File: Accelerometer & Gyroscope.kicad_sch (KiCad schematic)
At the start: 5 parts, among them U9 LSM6DS3

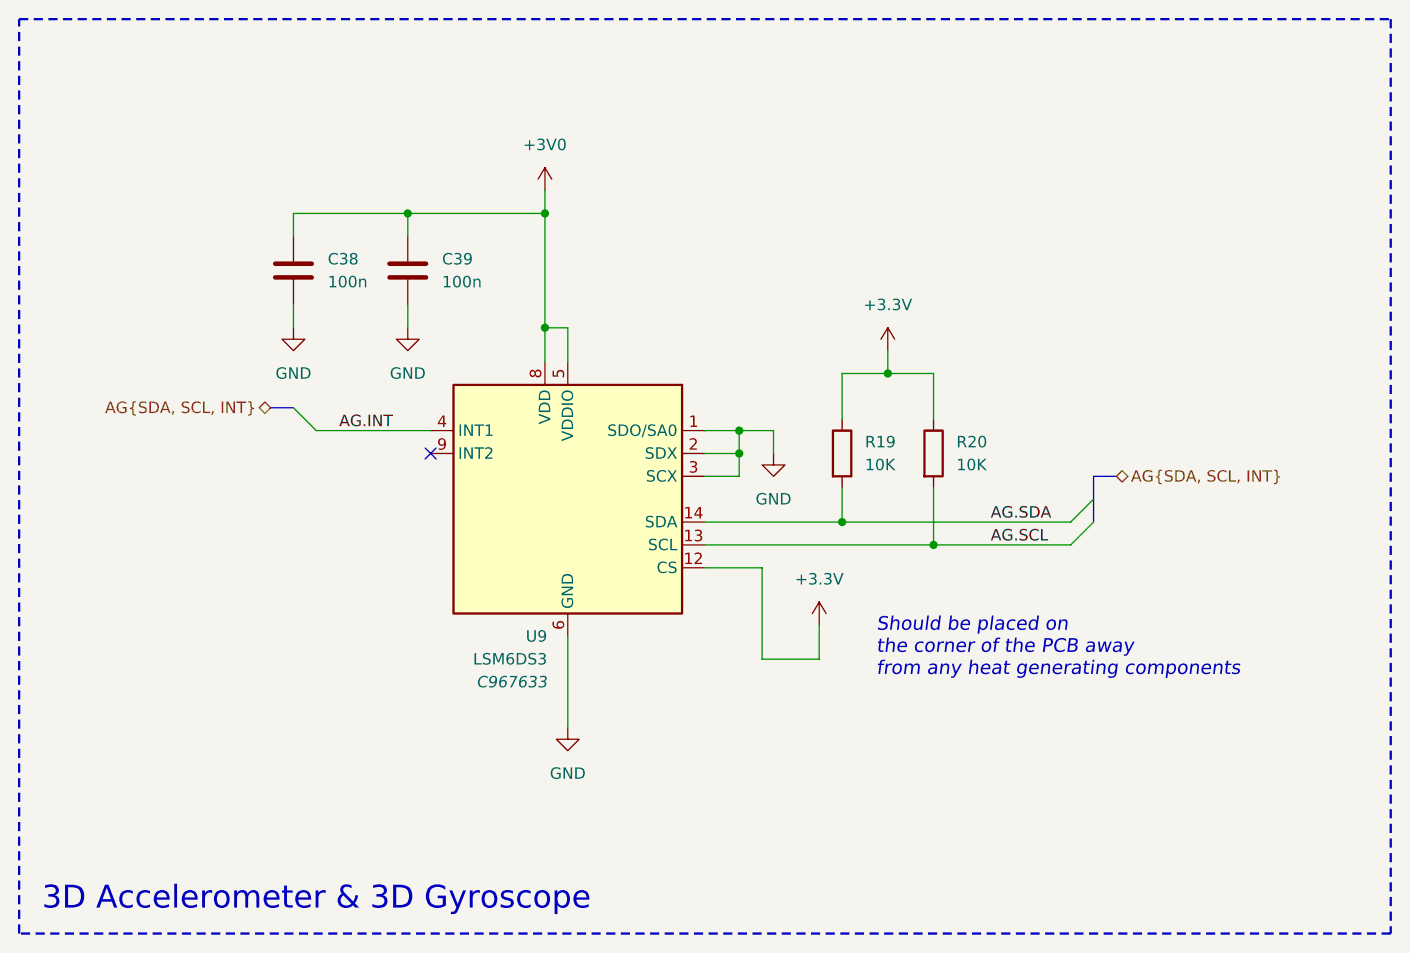
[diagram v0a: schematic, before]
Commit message: Pin out completion
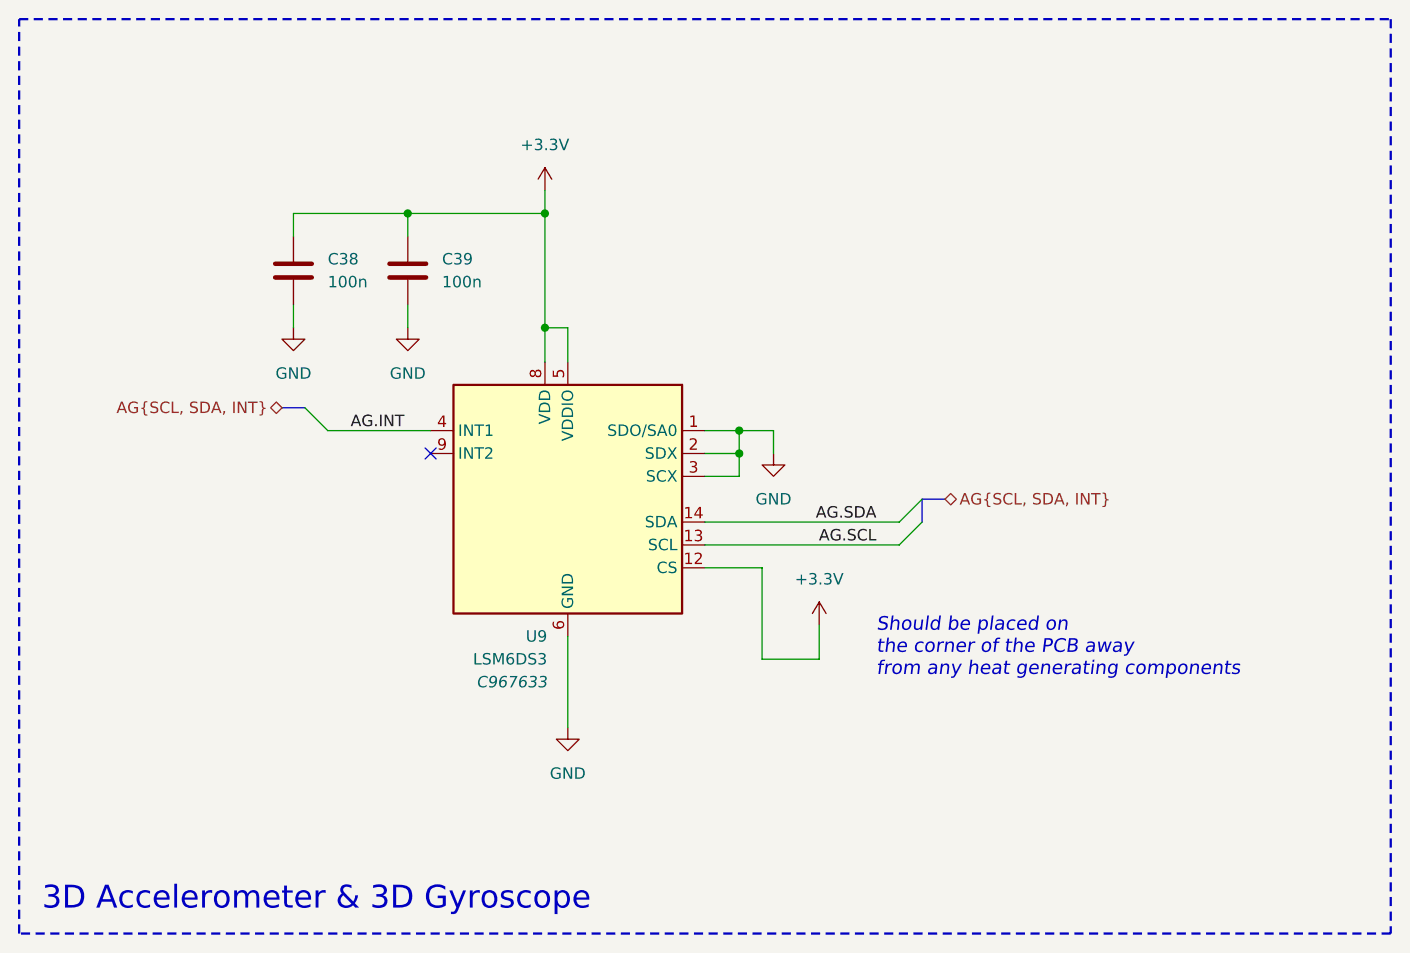
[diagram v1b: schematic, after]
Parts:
- removed R19, R20: 10K, Resistor_SMD:R_0402_1005Metric, symbol Device:R
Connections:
- net +3V0 is gone; now on net +3.3V: C38.1, C39.1, U9.5 (VDDIO), U9.8 (VDD)
